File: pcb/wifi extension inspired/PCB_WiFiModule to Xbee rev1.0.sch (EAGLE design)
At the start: 20 parts, among them J1 FA12-1W, U1 XBP9B-DMUT-002

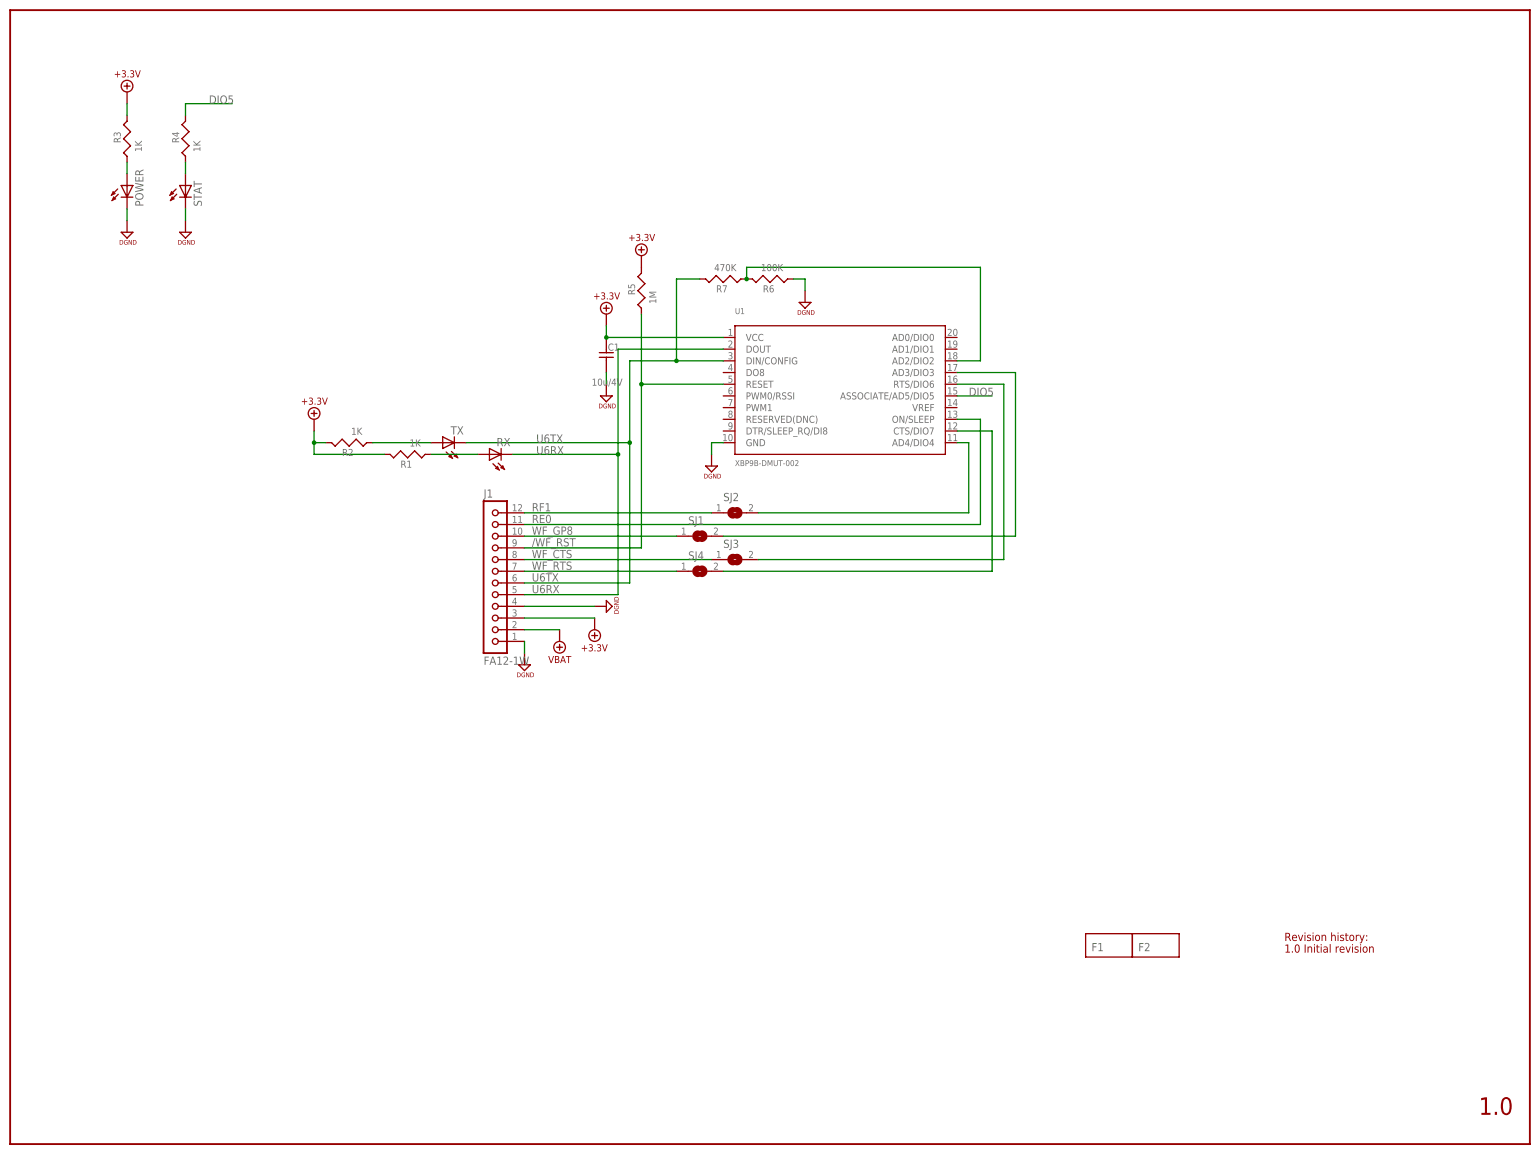
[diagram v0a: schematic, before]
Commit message: rev1.0 ready for review.
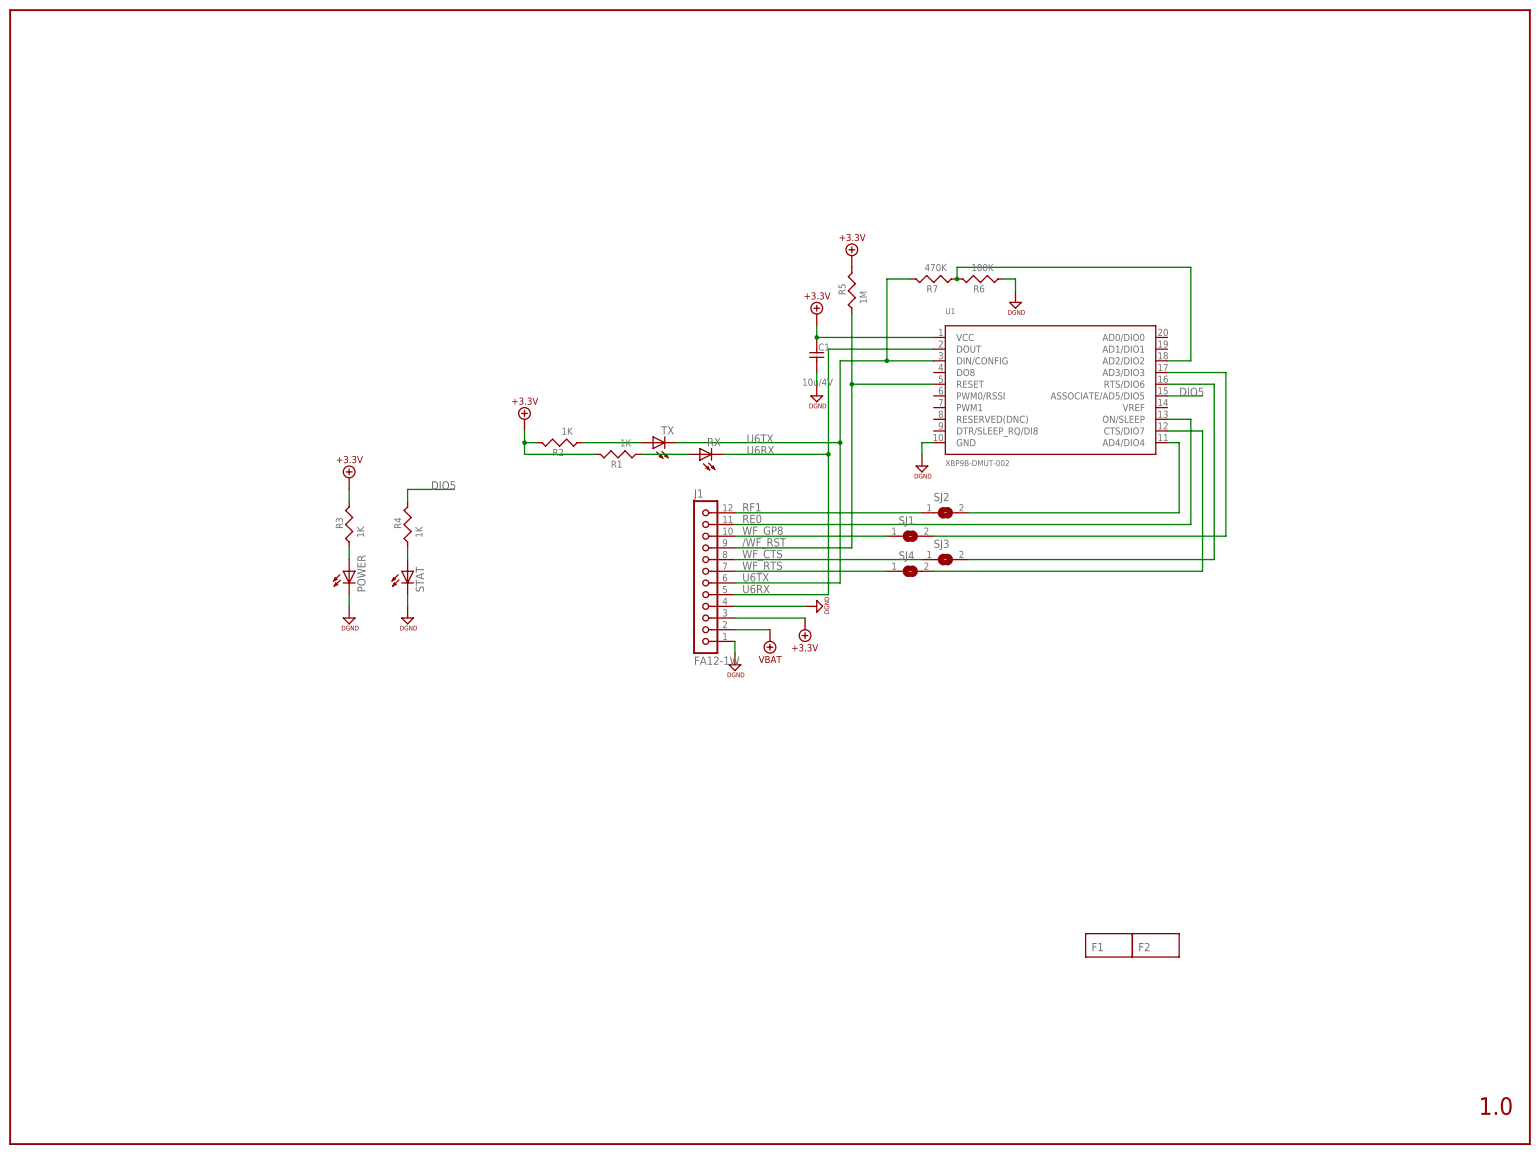
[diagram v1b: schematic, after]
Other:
- note removed: "1.0 Initial revision"
- note removed: "Revision history:"
- moved on the sheet: C1, J1, POWER, R1, R2, R3, R4, R5, R6, R7, RX, SJ1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
